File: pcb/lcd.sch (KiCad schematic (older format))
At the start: 1 part, among them U100 MCIMX7S5EVM08SC

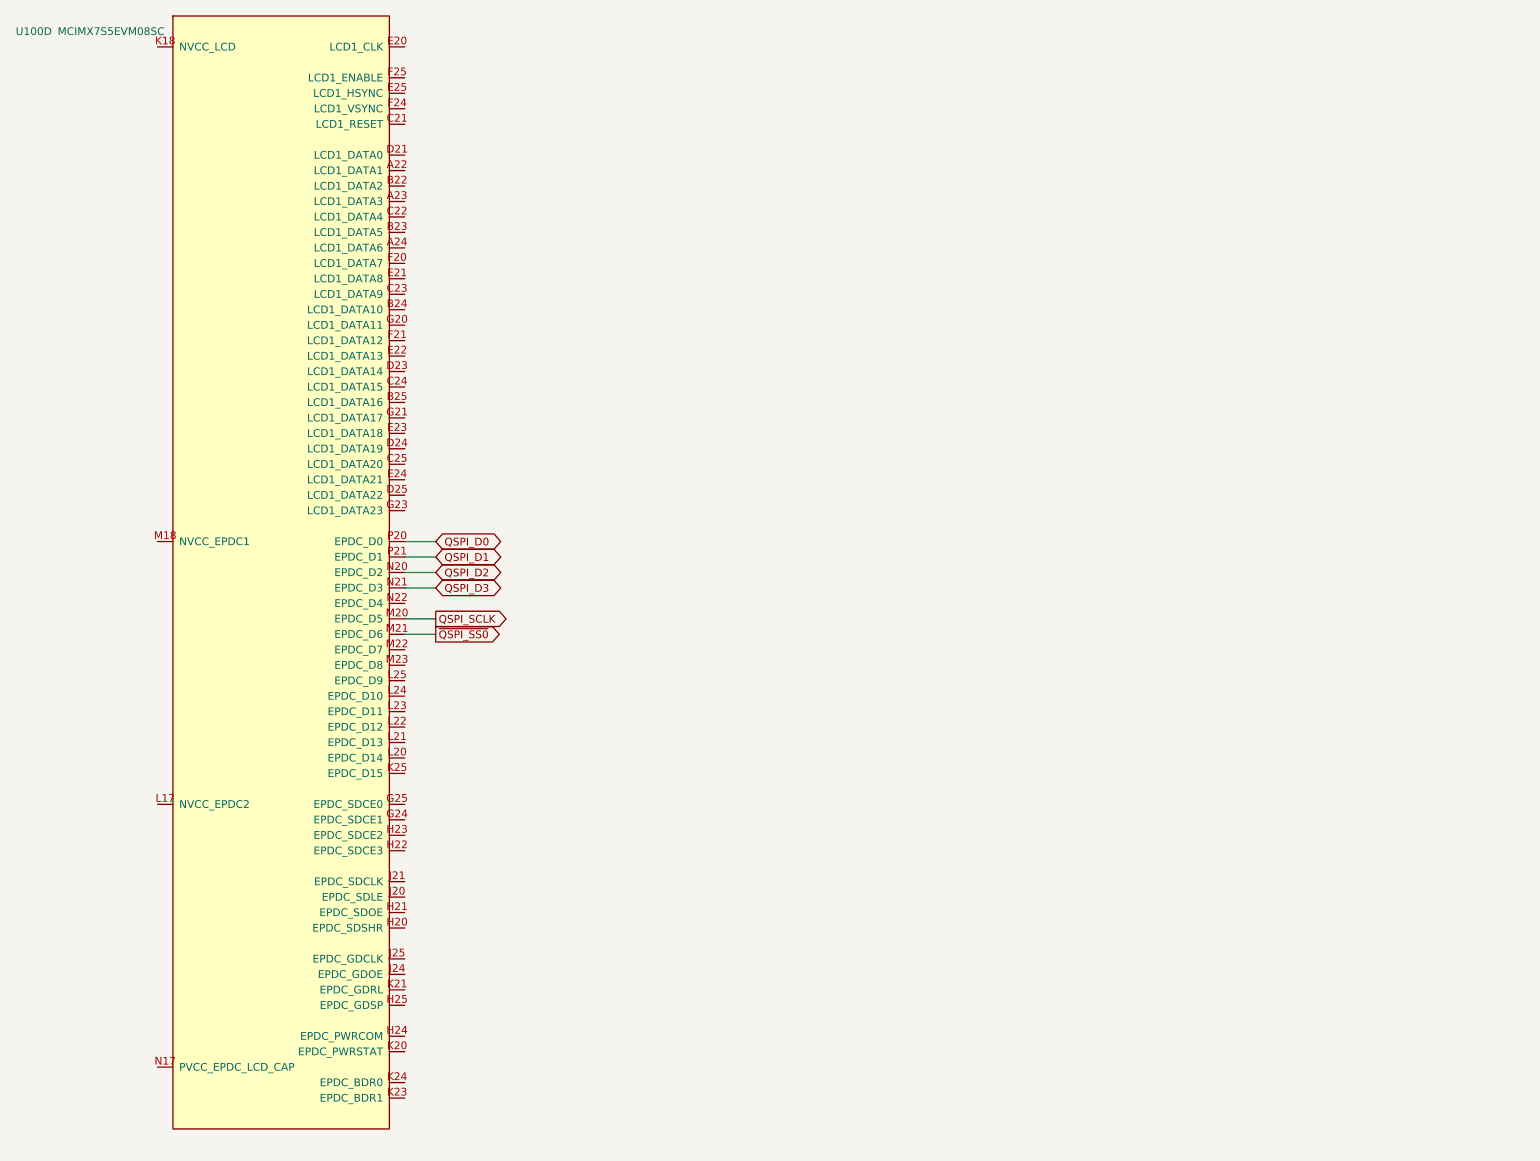
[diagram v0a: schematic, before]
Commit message: pcb: working on sch
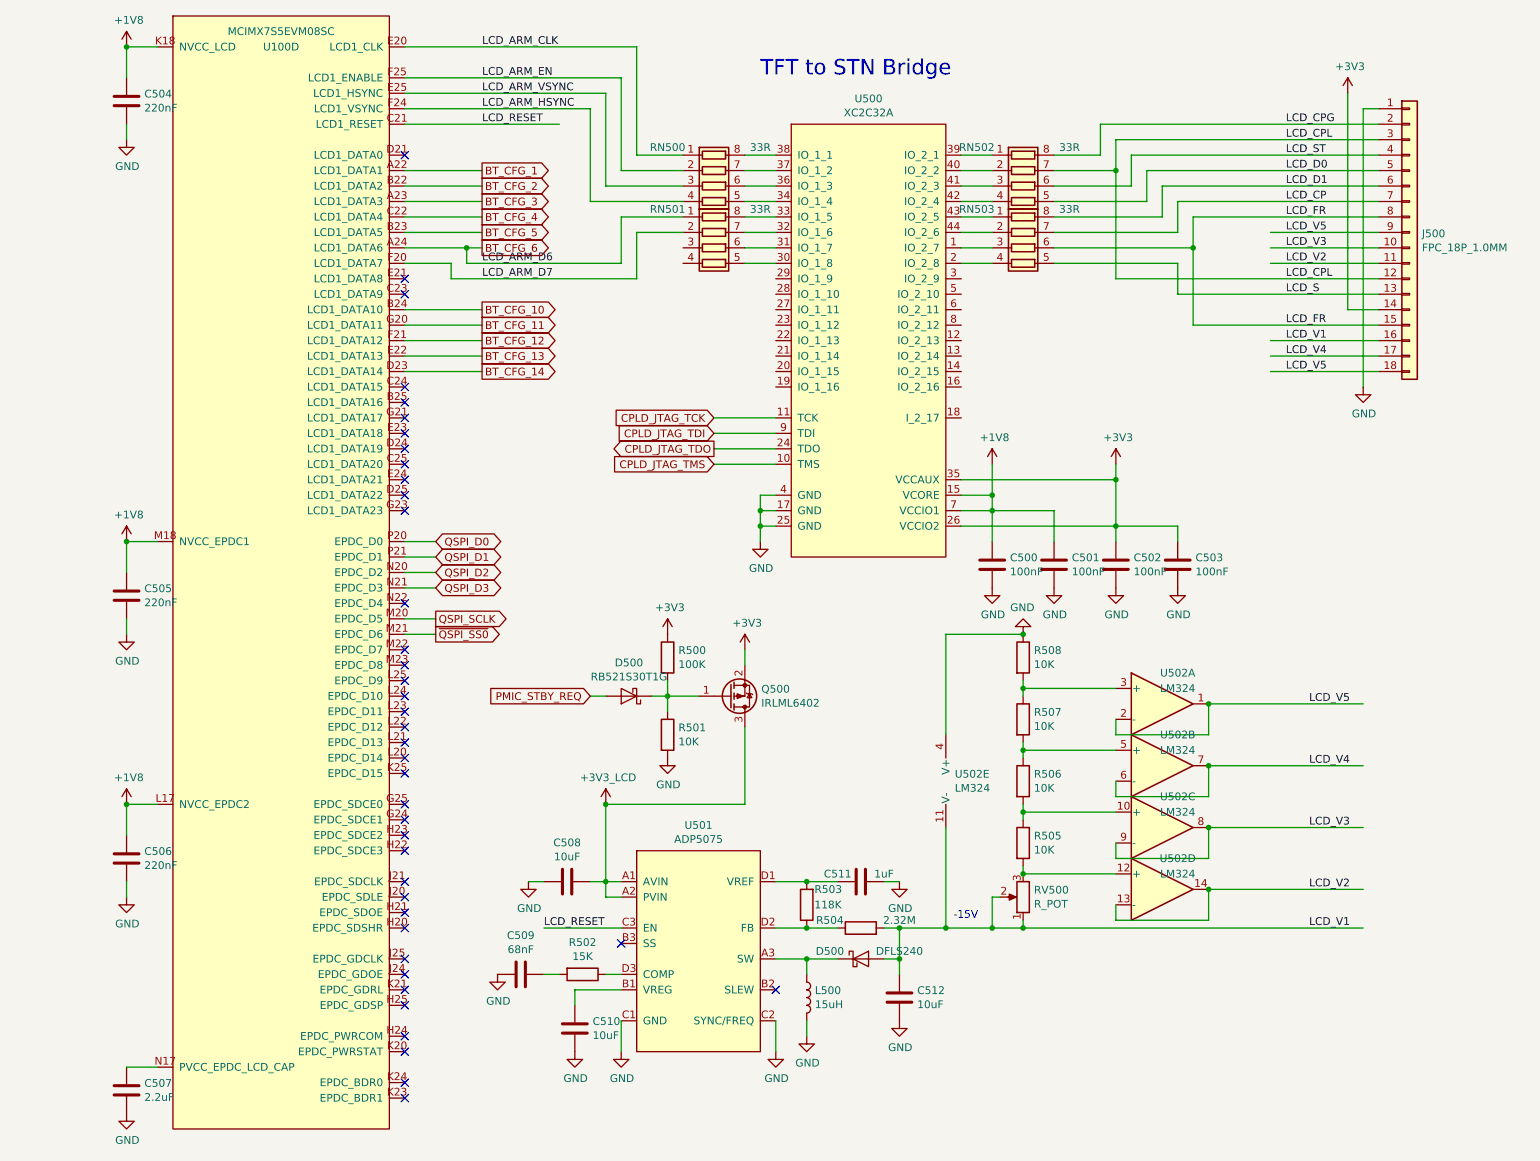
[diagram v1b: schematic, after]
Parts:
- added C500, C501, C502, C503: 100nF, symbol Device:C
- added C504, C505, C506: 220nF, symbol Device:C
- added C507: 2.2uF, symbol Device:C
- added C508, C510, C512: 10uF, symbol Device:C
- added C509: 68nF, symbol Device:C
- added C511: 1uF, symbol Device:C
- added D500: RB521S30T1G, symbol Device:D_Schottky
- added D500: DFLS240, symbol Device:D_Schottky
- added J500: FPC_18P_1.0MM, symbol Connector_Generic:Conn_01x18
- added L500: 15uH, symbol Device:L
- added Q500: IRLML6402, Package_TO_SOT_SMD:SOT-23, symbol Transistor_FET:IRLML6402
- added R500: 100K, symbol Device:R
- added R501, R505, R506, R507, R508: 10K, symbol Device:R
- added R502: 15K, symbol Device:R
- added R503: 118K, symbol Device:R
- added R504: 2.32M, symbol Device:R
- added RN500, RN501, RN502, RN503: 33R, symbol Device:R_Pack04
- added RV500: R_POT, symbol Device:R_POT
- added U500: XC2C32A, Package_QFP:LQFP-44_10x10mm_P0.8mm, symbol symbols:XC2C32A
- added U501: ADP5075, symbol symbols:ADP5075
- added U502: LM324, symbol Amplifier_Operational:LM324
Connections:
- net labels added: +1V8, +3V3, +3V3_LCD, BT_CFG_1, BT_CFG_10, BT_CFG_11, BT_CFG_12, BT_CFG_13, BT_CFG_14, BT_CFG_2, BT_CFG_3, BT_CFG_4, BT_CFG_5, BT_CFG_6, CPLD_JTAG_TCK, CPLD_JTAG_TDI, CPLD_JTAG_TDO, CPLD_JTAG_TMS, GND, LCD_ARM_CLK, LCD_ARM_D6, LCD_ARM_D7, LCD_ARM_EN, LCD_ARM_HSYNC, LCD_ARM_VSYNC, LCD_CP, LCD_CPG, LCD_CPL, LCD_D0, LCD_D1, LCD_FR, LCD_RESET, LCD_S, LCD_ST, LCD_V1, LCD_V2, LCD_V3, LCD_V4, LCD_V5, PMIC_STBY_REQ
- wire segments 6 -> 199
- no-connect marks 0 -> 40
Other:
- note added: "-15V"
- note added: "TFT to STN Bridge"
